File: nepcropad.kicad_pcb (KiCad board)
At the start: 2 copper layers, 58.7 x 65.2 mm, 36 parts, among them J1 USB_C_Receptacle_USB2.0, SW1 SW_Push, U1 ATmega32U4-A, Y1 16MHz

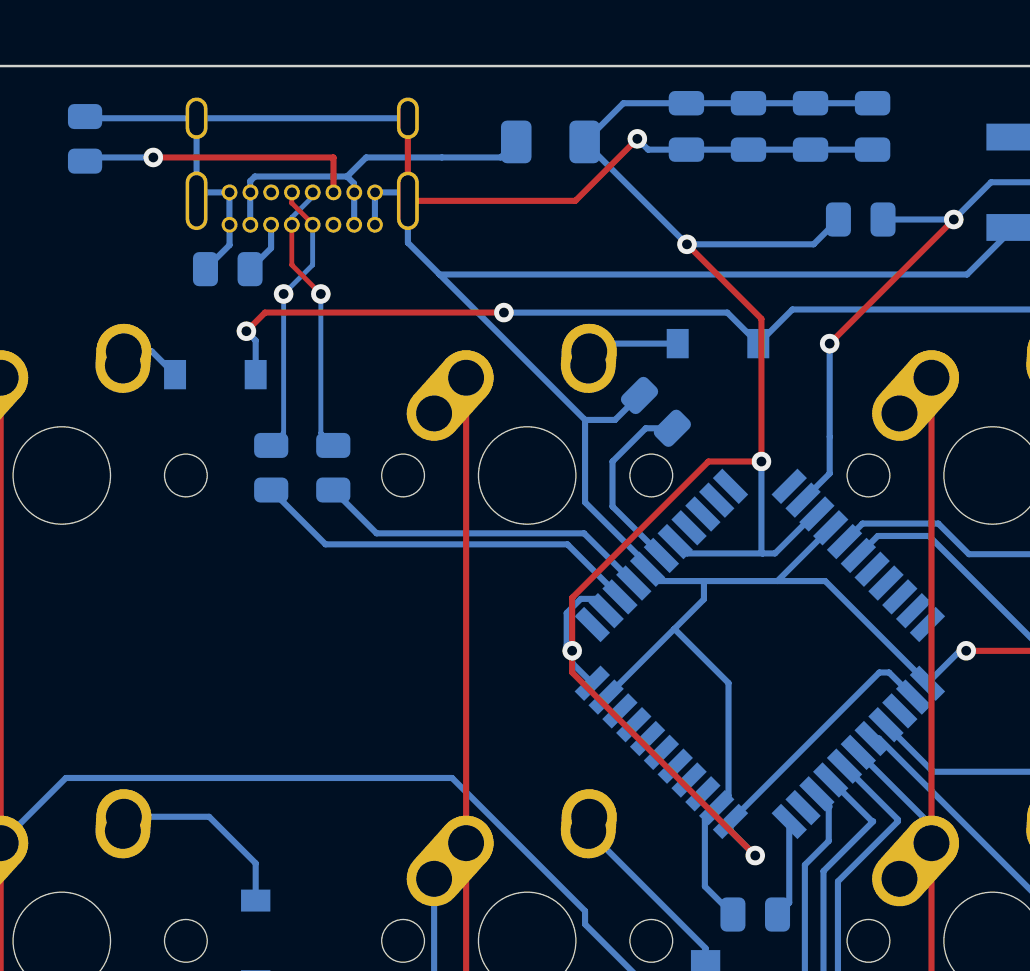
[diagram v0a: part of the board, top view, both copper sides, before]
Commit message: cleanup
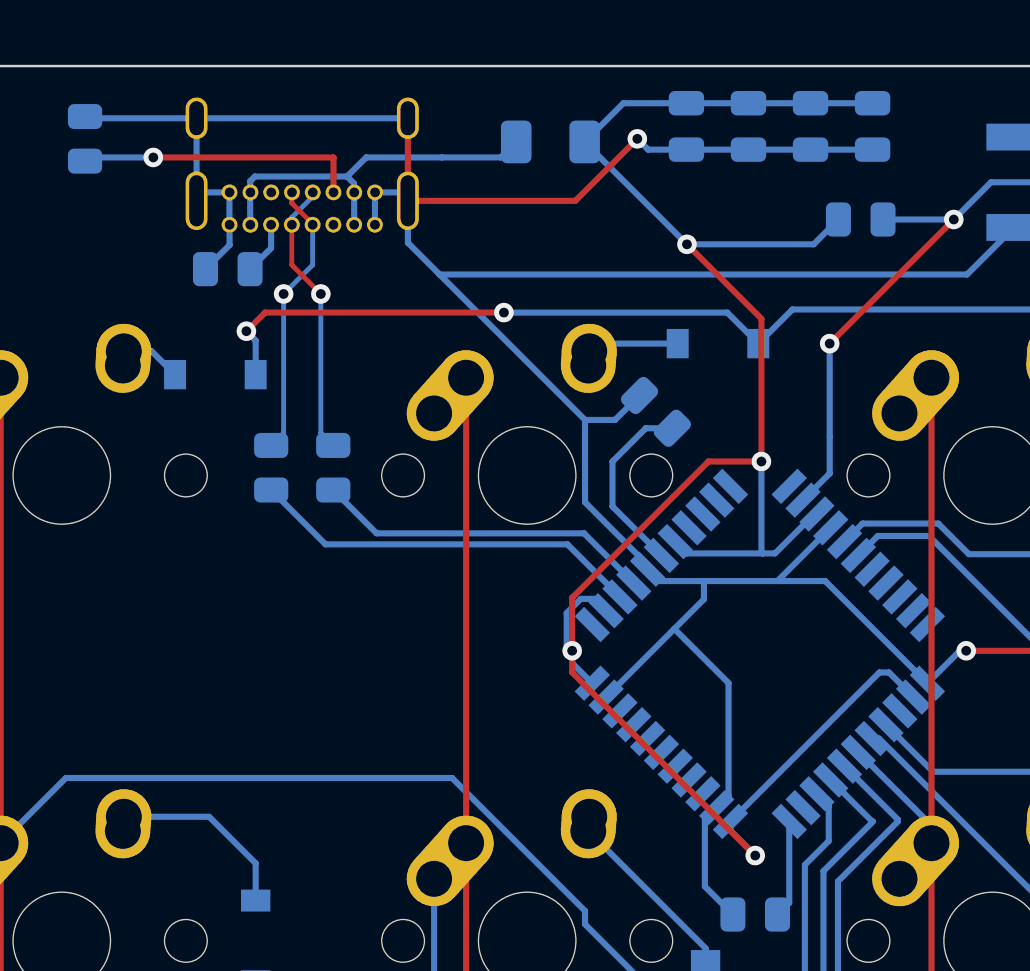
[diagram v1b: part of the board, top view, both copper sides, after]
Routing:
- net COL0: track 85.7 -> 85.0 mm
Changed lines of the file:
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@@
   (segment (start 160.011508 77.715508) (end 157.21925 80.507767) (width 0.25) (layer "B.Cu") (net 1))
   (segment (start 179.319 76.581) (end 179.596 76.858) (width 0.25) (layer "B.Cu") (net 1))
-  (segment (start 168.12569 58.1) (end 168.43569 58.1) (width 0.25) (layer "B.Cu") (net 1))
   (segment (start 141.805 61.175) (end 141.805 62.0065) (width 0.25) (layer "B.Cu") (net 1))
   (segment (start 161.222725 75.759275) (end 164.230483 75.759275) (width 0.25) (layer "B.Cu") (net 1))
@@
   (segment (start 158.840249 69.505751) (end 159.929751 69.505751) (width 0.25) (layer "B.Cu") (net 4))
   (segment (start 160.528 61.976) (end 163.576 65.024) (width 0.25) (layer "F.Cu") (net 5))
-  (segment (start 160.528 61.976) (end 160.528 61.788) (width 0.25) (layer "F.Cu") (net 5))
   (segment (start 163.576 70.866) (end 161.406769 70.866) (width 0.25) (layer "F.Cu") (net 5))
   (segment (start 155.829 79.502) (end 155.829 78.613) (width 0.25) (layer "F.Cu") (net 5))
@@
   (segment (start 165.354 92.71) (end 159.258 92.71) (width 0.25) (layer "B.Cu") (net 19))
   (segment (start 156.356401 89.262861) (end 150.91354 83.82) (width 0.25) (layer "B.Cu") (net 19))
-  (segment (start 165.845952 84.467565) (end 166.37 84.991613) (width 0.25) (layer "B.Cu") (net 19))
   (segment (start 165.354 87.376) (end 165.354 92.71) (width 0.25) (layer "B.Cu") (net 19))
   (segment (start 166.330051 84.951664) (end 166.330051 86.399949) (width 0.25) (layer "B.Cu") (net 19))
@@
   (segment (start 166.411638 83.90188) (end 168.107758 85.598) (width 0.25) (layer "B.Cu") (net 20))
   (segment (start 166.116 87.63) (end 166.116 93.472) (width 0.25) (layer "B.Cu") (net 20))
-  (segment (start 168.107758 85.598) (end 168.148 85.598) (width 0.25) (layer "B.Cu") (net 20))
   (segment (start 150.1775 93.0275) (end 150.1775 87.9475) (width 0.25) (layer "B.Cu") (net 20))
   (segment (start 168.148 85.598) (end 166.116 87.63) (width 0.25) (layer "B.Cu") (net 20))
@@
   (segment (start 146.06 58.43) (end 146.05 58.42) (width 0.25) (layer "F.Cu") (net 49))
   (via (at 138.684 58.42) (size 0.8) (drill 0.4) (layers "F.Cu" "B.Cu") (net 49))
-  (segment (start 138.5335 58.5705) (end 138.684 58.42) (width 0.25) (layer "B.Cu") (net 49))
   (segment (start 136.0405 58.42) (end 135.89 58.5705) (width 0.25) (layer "B.Cu") (net 49))
   (segment (start 138.684 58.42) (end 136.0405 58.42) (width 0.25) (layer "B.Cu") (net 49))
